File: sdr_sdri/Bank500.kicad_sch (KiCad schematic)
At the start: 4 parts

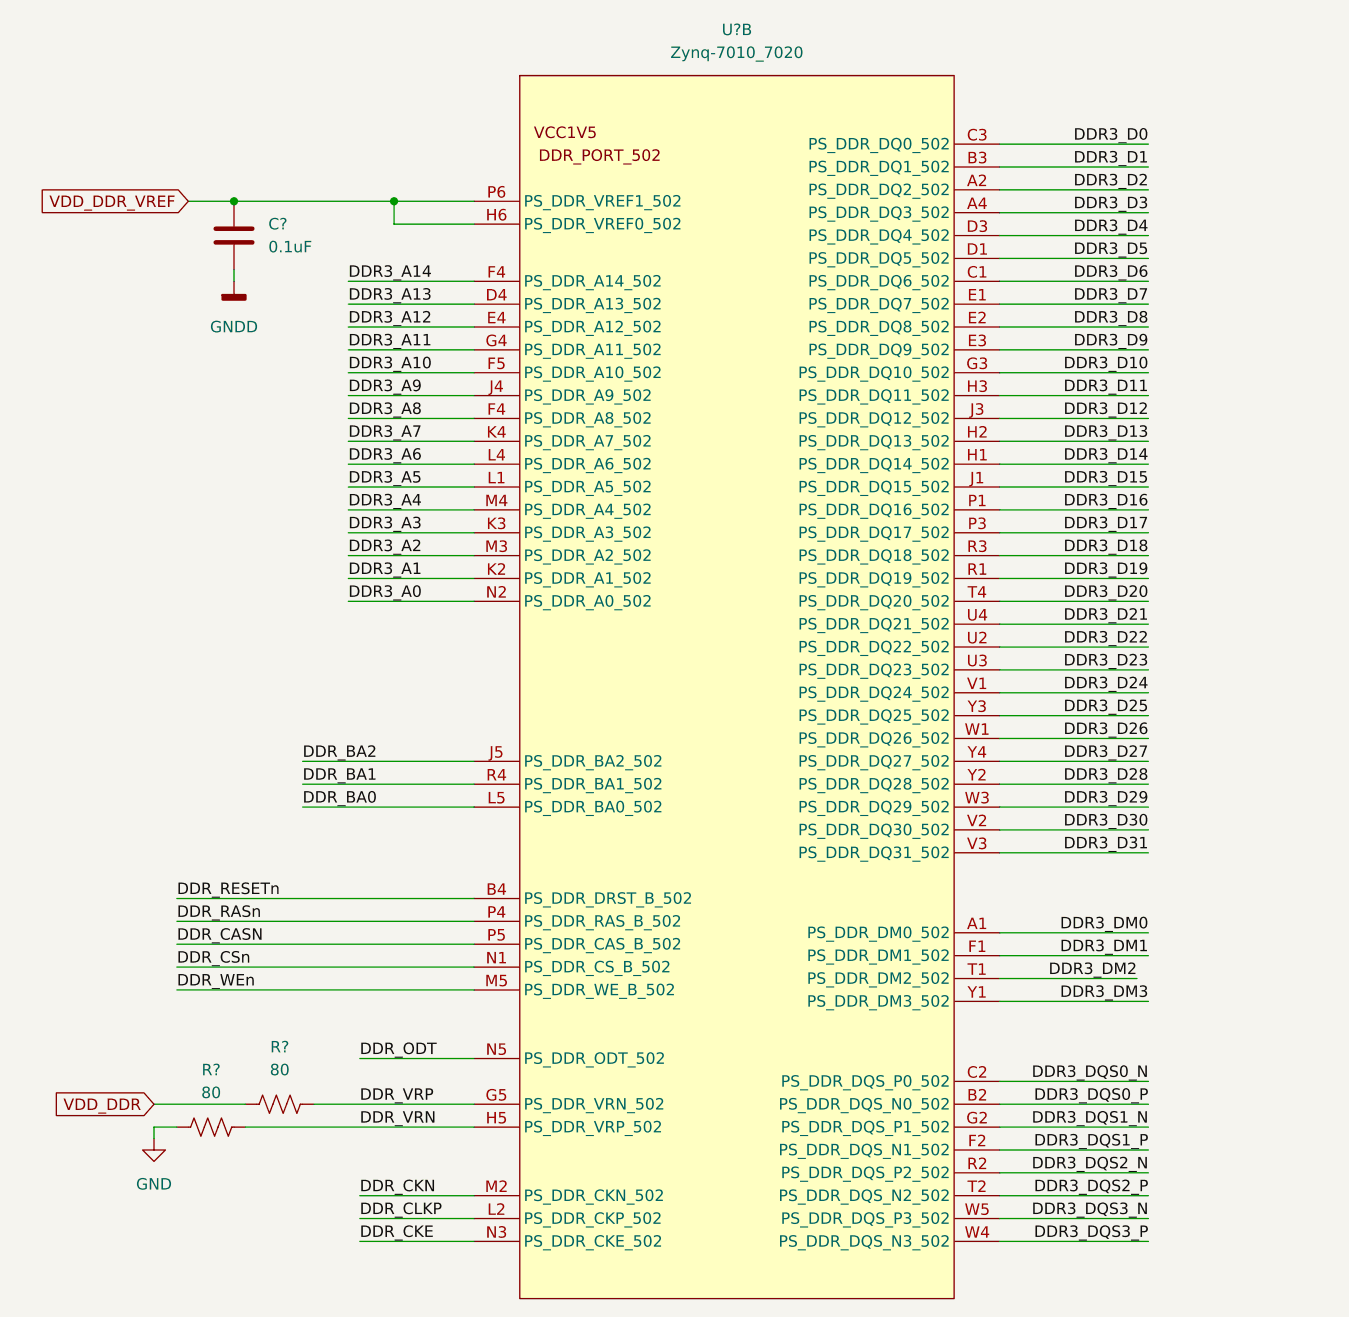
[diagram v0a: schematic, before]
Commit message: menambahkan connecsi k
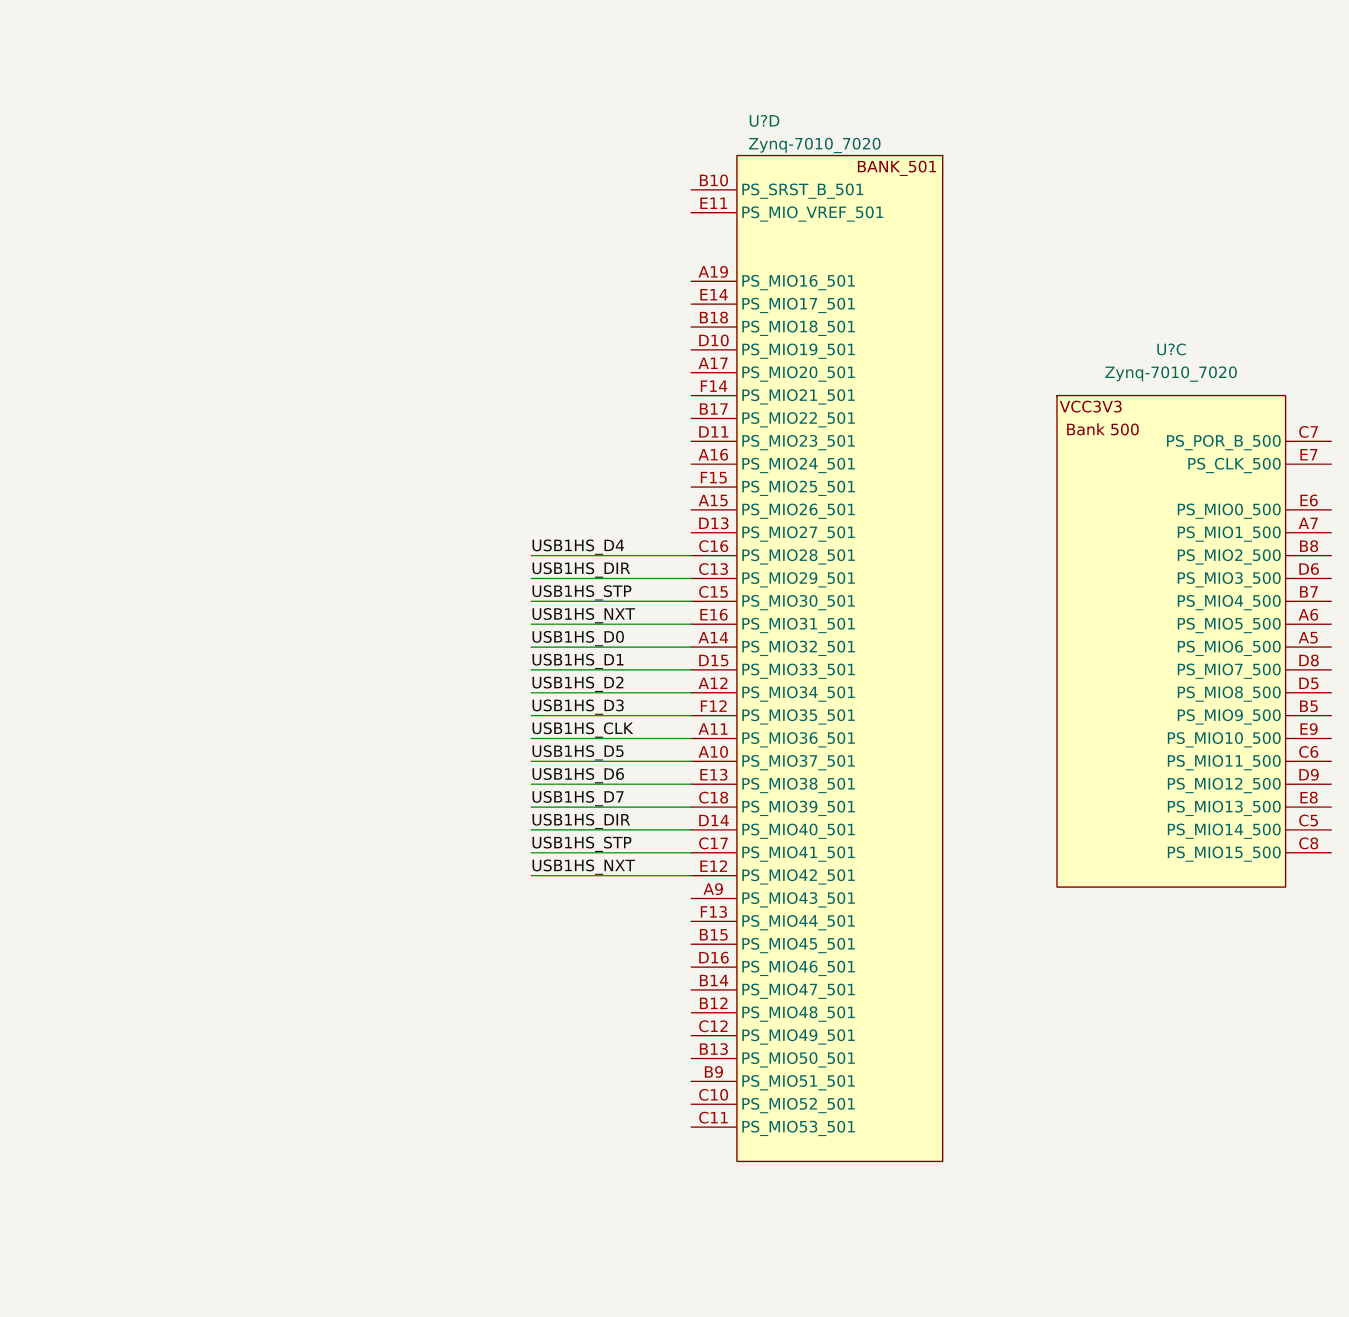
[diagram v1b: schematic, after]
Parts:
- removed C?: 0.1uF, symbol Device:C
- removed R? (x2): 80, symbol Device:R_US
- removed U?: Zynq-7010_7020, symbol Zynq7000:Zynq-7010_7020
- added U? (x2): Zynq-7010_7020, symbol Zynq7000:Zynq-7010_7020
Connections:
- new net USB1HS_CLK: U?.A11 (PS_MIO36_501)
- new net USB1HS_D0: U?.A14 (PS_MIO32_501)
- new net USB1HS_D1: U?.D15 (PS_MIO33_501)
- new net USB1HS_D2: U?.A12 (PS_MIO34_501)
- new net USB1HS_D3: U?.F12 (PS_MIO35_501)
- new net USB1HS_D4: U?.C16 (PS_MIO28_501)
- new net USB1HS_D5: U?.A10 (PS_MIO37_501)
- new net USB1HS_D6: U?.E13 (PS_MIO38_501)
- new net USB1HS_D7: U?.C18 (PS_MIO39_501)
- new net USB1HS_DIR: U?.C13 (PS_MIO29_501), U?.D14 (PS_MIO40_501)
- new net USB1HS_NXT: U?.E12 (PS_MIO42_501), U?.E16 (PS_MIO31_501)
- new net USB1HS_STP: U?.C15 (PS_MIO30_501), U?.C17 (PS_MIO41_501)
